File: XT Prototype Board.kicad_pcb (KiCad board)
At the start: 2 copper layers, 98.4 x 73.9 mm, 22 parts, among them J1 Bus_ISA_8bit, J2 Breakout, SW1 SW_DIP_x08, U1 AS6C4008-55PCN, U2 74LS151, U3 74LS245, U4 74LS02, U5 74LS00

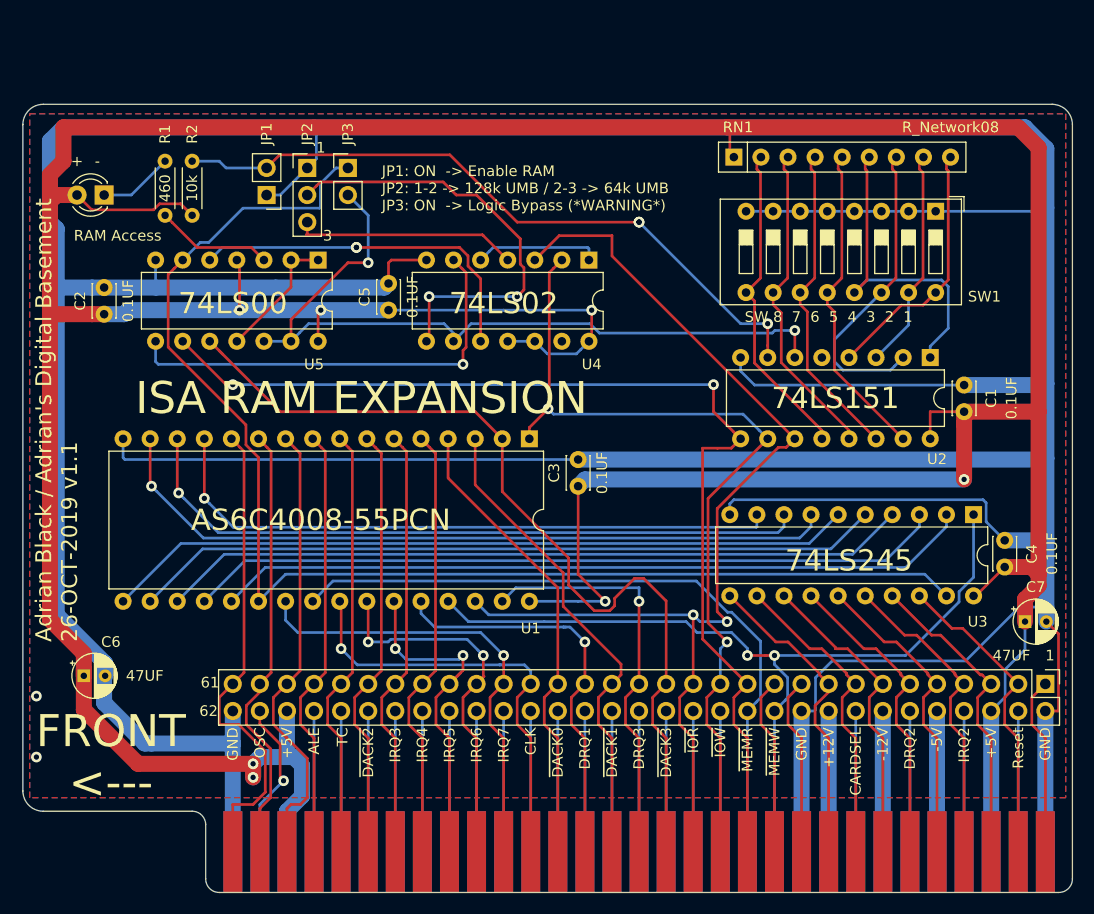
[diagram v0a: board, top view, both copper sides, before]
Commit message: Initial fix
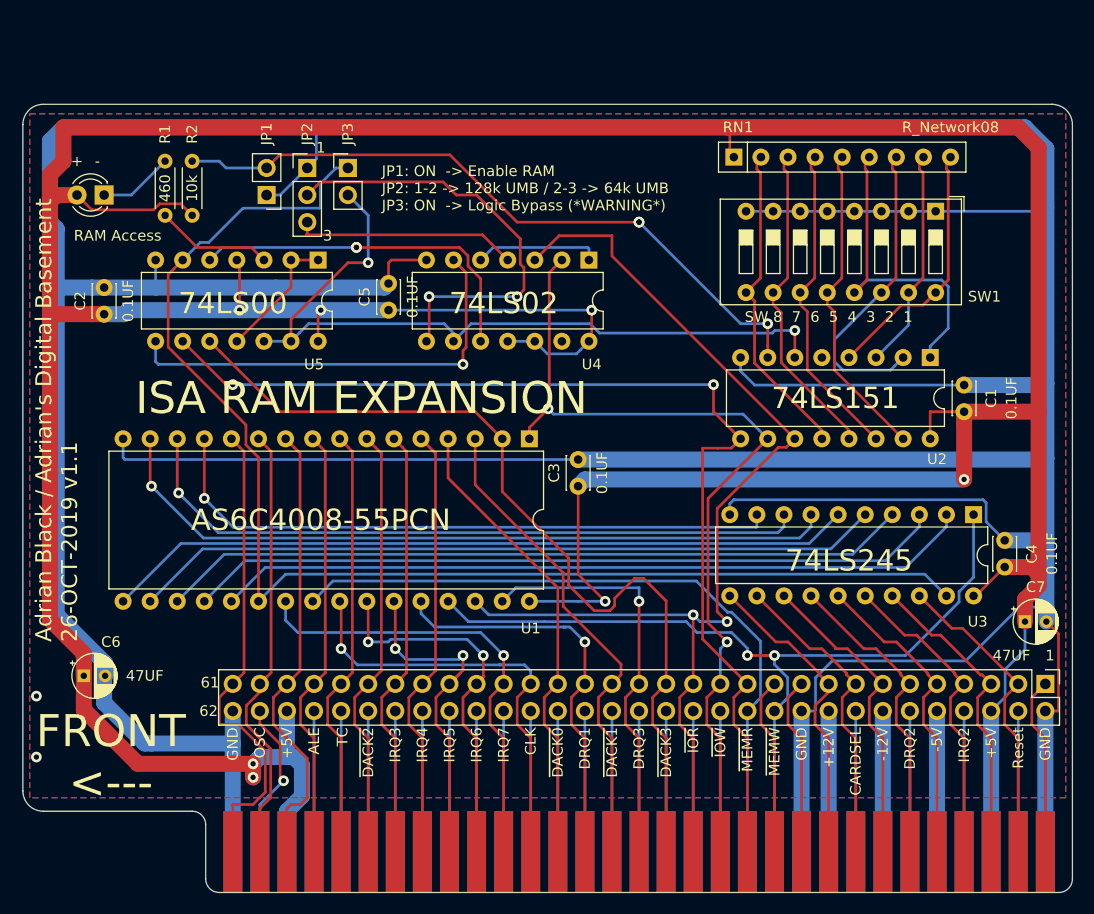
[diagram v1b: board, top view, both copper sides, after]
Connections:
- net ~DACK0 renamed ~{DACK0}
- net ~DACK1 renamed ~{DACK1}
- net ~DACK2 renamed ~{DACK2}
- net ~DACK3 renamed ~{DACK3}
- net ~IOR renamed ~{IOR}
- net ~IOW renamed ~{IOW}
- net ~MEMR renamed ~{MEMR}
- net ~MEMW renamed ~{MEMW}
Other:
- net class Default removed
- board text added: "~{DACK0}"
- board text added: "~{DACK1}"
- board text added: "~{DACK2}"
- board text added: "~{DACK3}"
- board text added: "~{IOR}"
- board text added: "~{IOW}"
- board text added: "~{MEMR}"
- board text added: "~{MEMW}"
- board text removed: "~DACK0"
- board text removed: "~DACK1"
- board text removed: "~DACK2"
- board text removed: "~DACK3"
- board text removed: "~IOR"
- board text removed: "~IOW"
- board text removed: "~MEMR"
- board text removed: "~MEMW"
